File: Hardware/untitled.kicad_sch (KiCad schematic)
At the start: 11 parts, among them J7 Solar panel input, U1 MCP16311

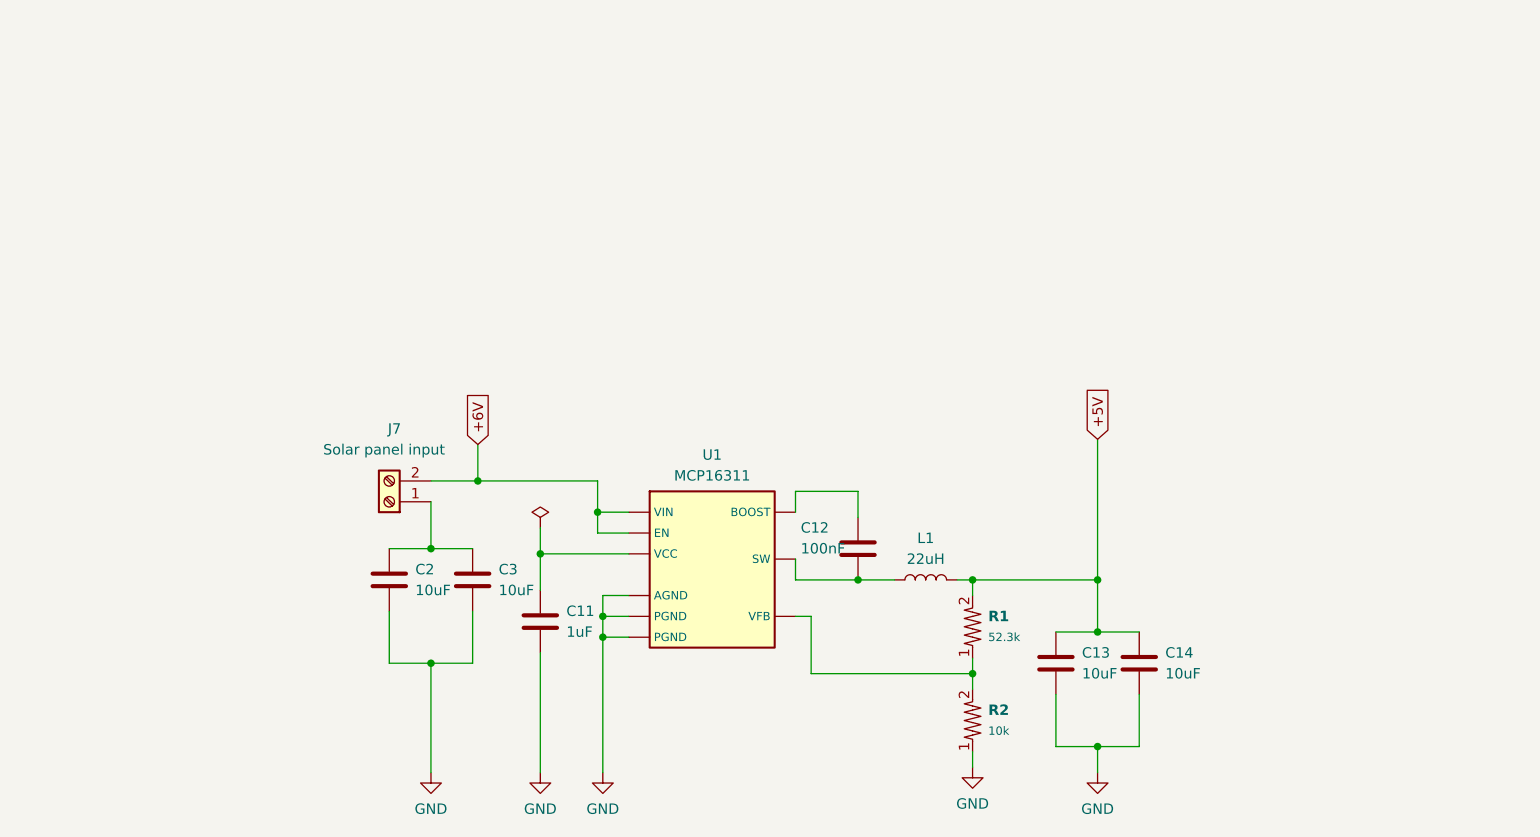
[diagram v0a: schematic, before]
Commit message: CHECK
CHECK1
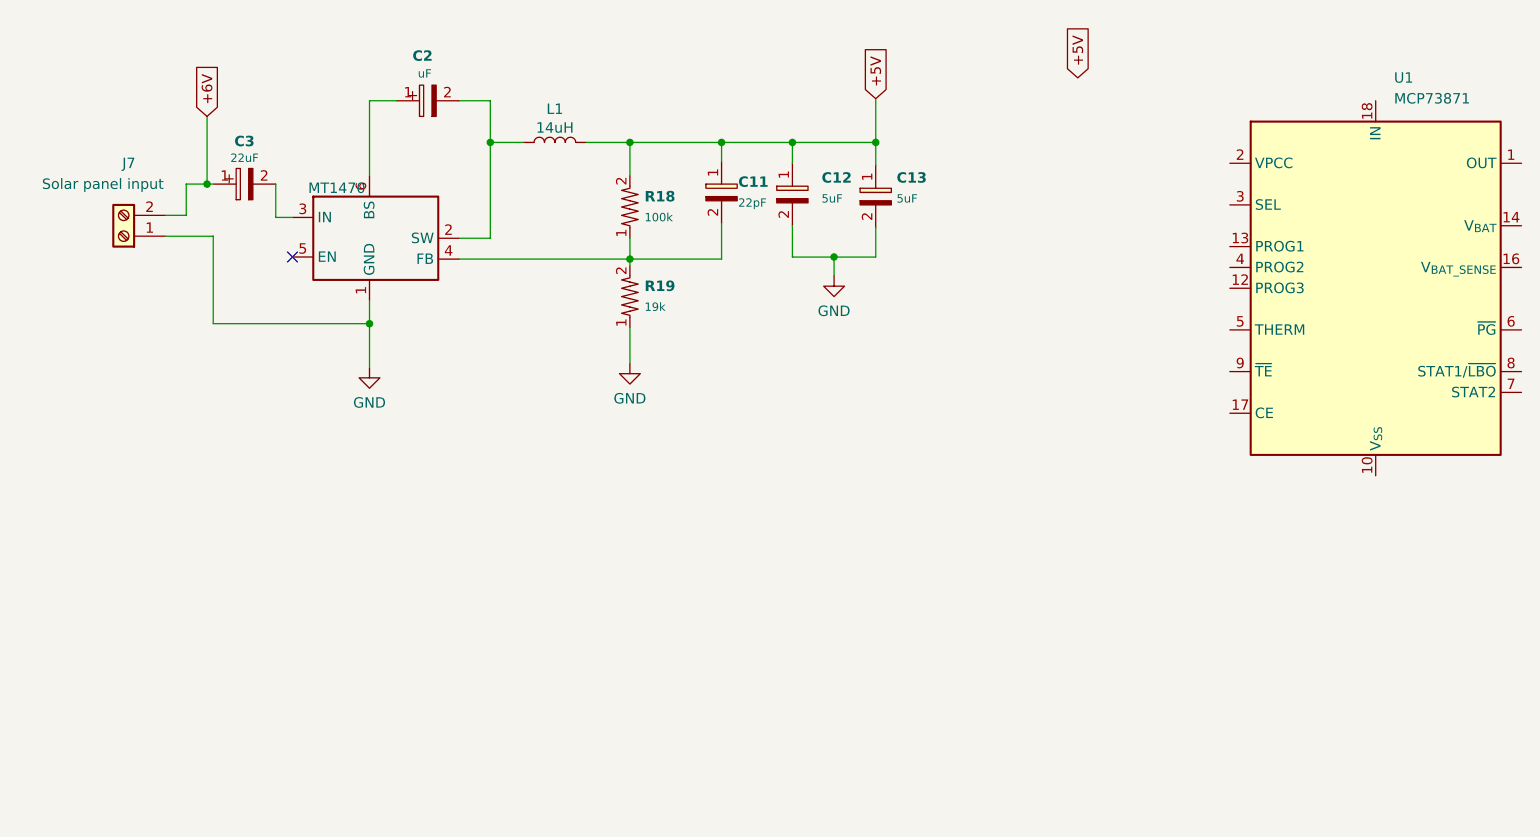
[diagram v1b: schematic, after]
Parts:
- removed C11: 1uF, symbol Device:C
- removed C12: 100nF, symbol Device:C
- removed C13, C14, C2, C3: 10uF, symbol Device:C
- removed R1: 52.3k, symbol Triet_KiCAD_Sym:Res
- removed R2: 10k, symbol Triet_KiCAD_Sym:Res
- removed U1: MCP16311, Triet_KiCAD_Fprint:MCP16311, symbol Triet_KiCAD_Sym:MCP16311
- added C11: 22pF, symbol Triet_KiCAD_Sym:CAP_CER
- added C12, C13: 5uF, symbol Triet_KiCAD_Sym:CAP_CER
- added C2: uF, symbol Triet_KiCAD_Sym:CAP_POL
- added C3: 22uF, symbol Triet_KiCAD_Sym:CAP_POL
- added MT1470: ~, symbol thinh:MT1470
- added R18: 100k, symbol Triet_KiCAD_Sym:Res
- added R19: 19k, symbol Triet_KiCAD_Sym:Res
- added U1: MCP73871, Package_DFN_QFN:QFN-20-1EP_4x4mm_P0.5mm_EP2.5x2.5mm, symbol Battery_Management:MCP73871
- L1: value 22uH -> 14uH
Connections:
- net +5V: now also C11.1, C12.1, C13.1, R18.2
- net +6V: now also C3.1
- net GND: now also J7.1 (Pin_1), C12.2, C13.2, MT1470.1 (GND), R19.1
- net at L1.1: now also C2.2, MT1470.2 (SW)
- new net: C3.2, MT1470.3 (IN)
- new net: C11.2, MT1470.4 (FB), R18.1, R19.2
- new net: C2.1, MT1470.6 (BS)
- new net: U1.1 (OUT), U1.20 (OUT)
- new net: U1.10 (V_{SS}), U1.11 (V_{SS}), U1.21 (V_{SS})
- new net: U1.14 (V_{BAT}), U1.15 (V_{BAT})
- new net: U1.18 (IN), U1.19 (IN)
- no-connect marks 0 -> 1
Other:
- moved on the sheet: J7

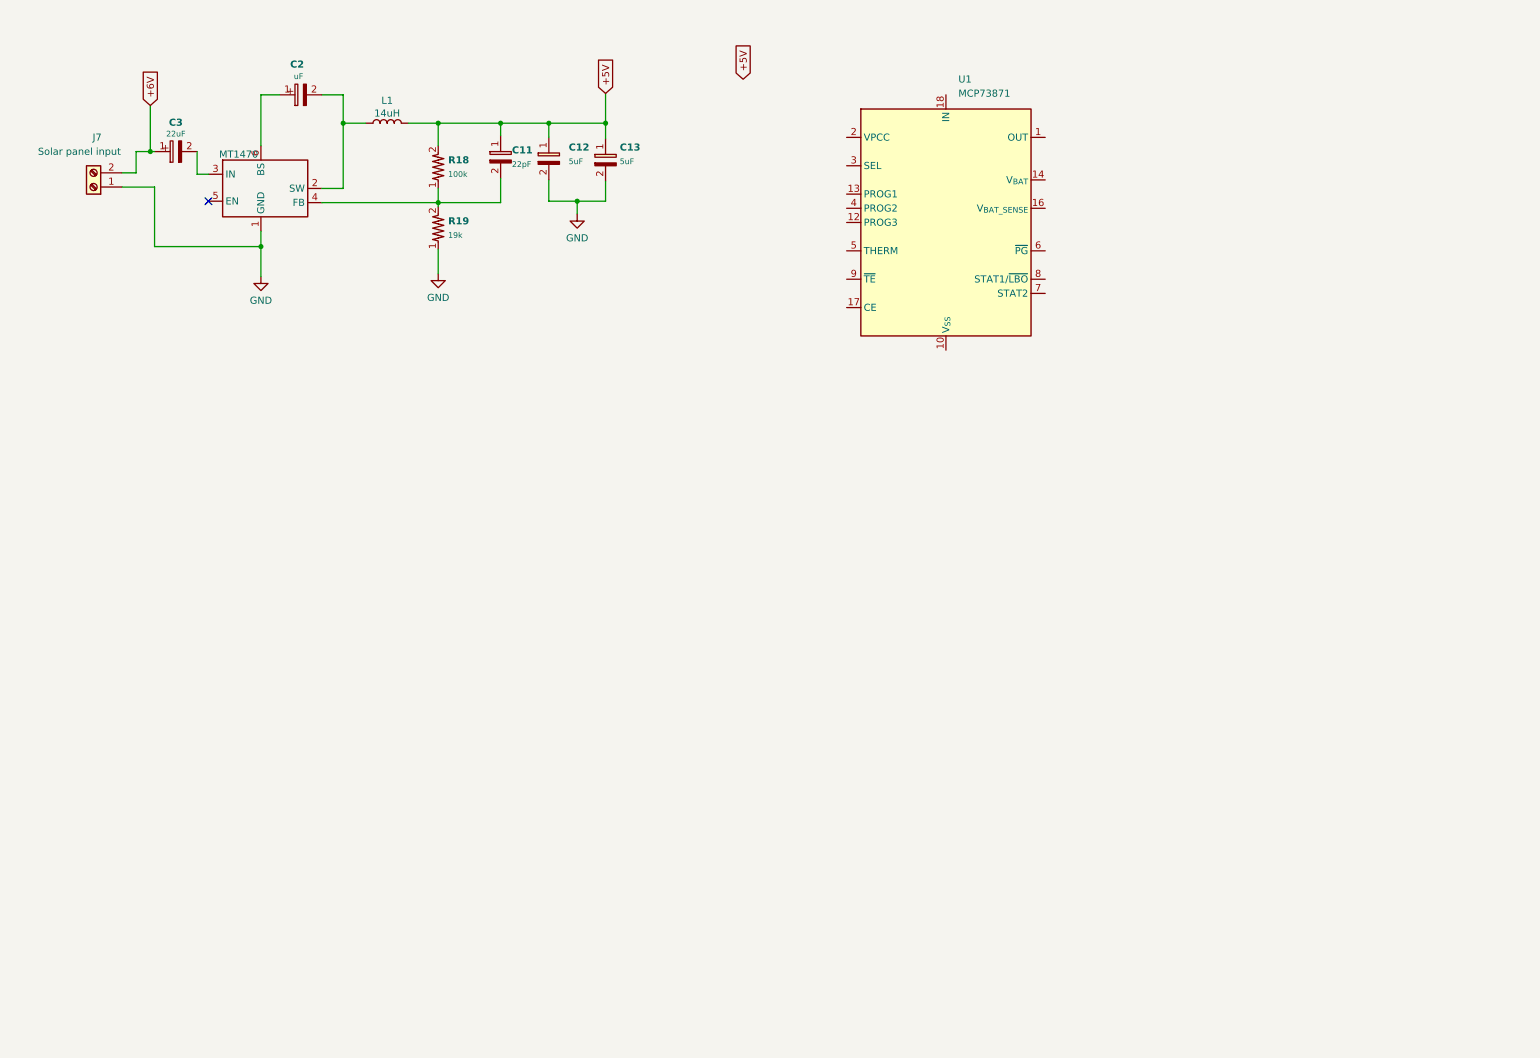
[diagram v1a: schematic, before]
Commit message: CHECK
CHECK
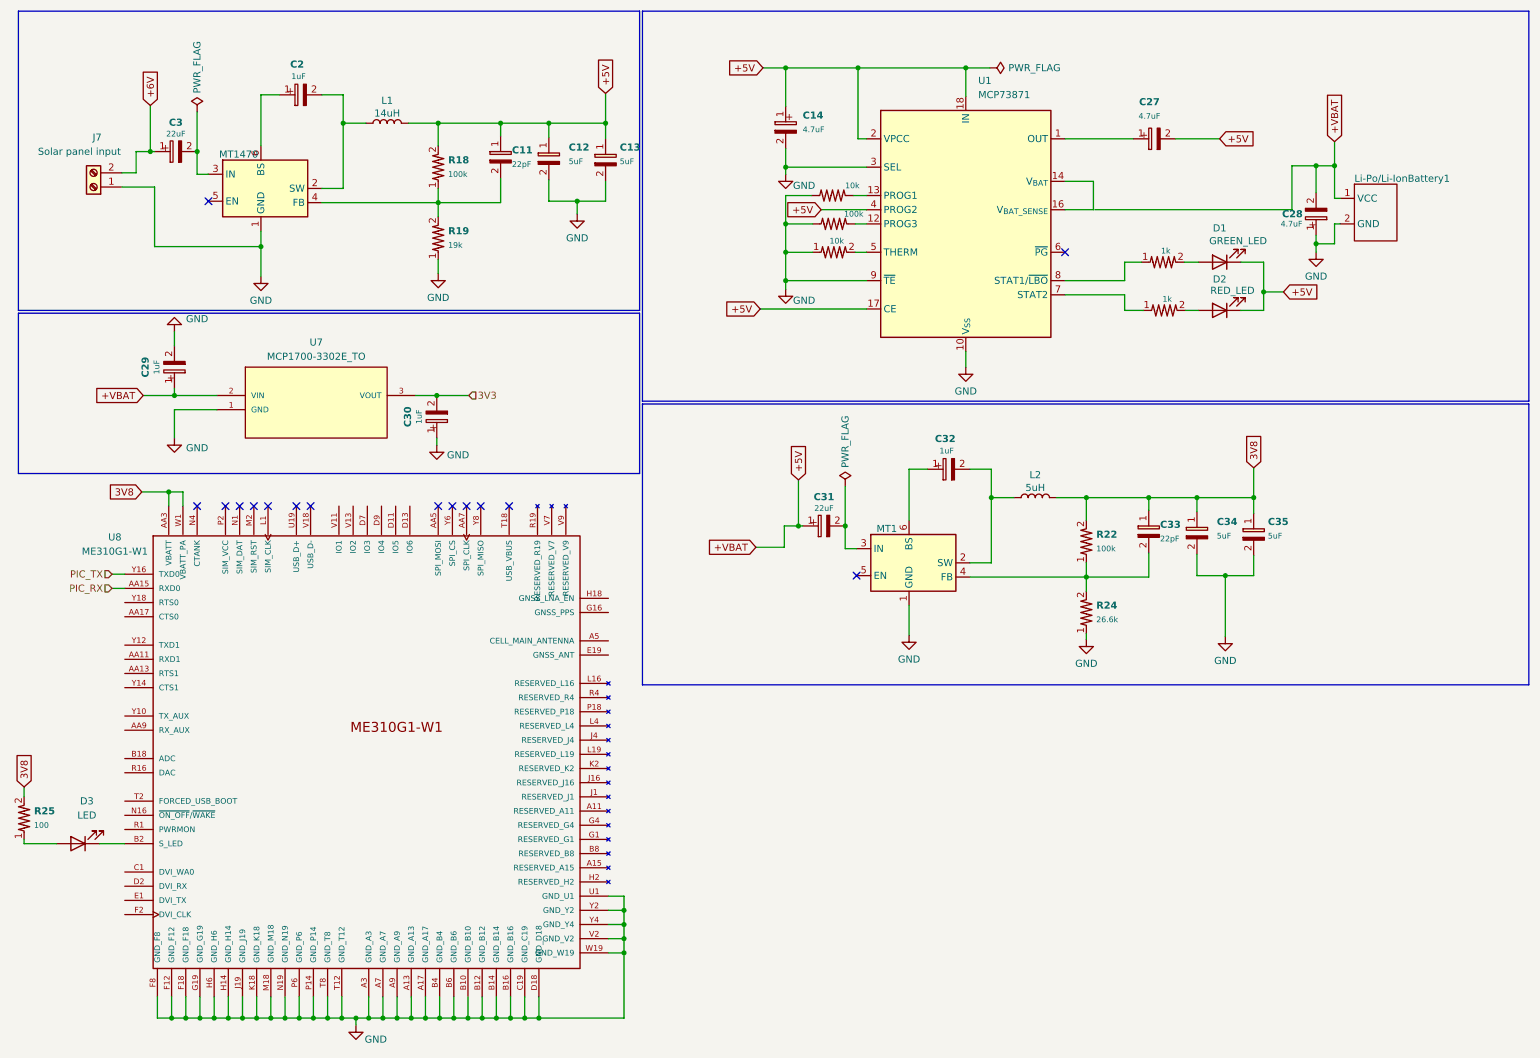
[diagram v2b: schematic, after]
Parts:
- added C14, C27, C28: 4.7uF, symbol Triet_KiCAD_Sym:CAP_POL
- added C29, C30, C32: 1uF, symbol Triet_KiCAD_Sym:CAP_POL
- added C31: 22uF, symbol Triet_KiCAD_Sym:CAP_POL
- added C33: 22pF, symbol Triet_KiCAD_Sym:CAP_CER
- added C34, C35: 5uF, symbol Triet_KiCAD_Sym:CAP_CER
- added D1: GREEN_LED, symbol Device:LED
- added D2: RED_LED, symbol Device:LED
- added D3: LED, symbol Device:LED
- added L2: 5uH, symbol Device:L
- added Li-Po/Li-IonBattery1: ~, symbol thinh:Li-Po/Li-Ion_Battery
- added MT1: ~, symbol thinh:MT1470
- added R17, R21: 1k, symbol Triet_KiCAD_Sym:Res
- added R2, R22: 100k, symbol Triet_KiCAD_Sym:Res
- added R20, R23: 10k, symbol Triet_KiCAD_Sym:Res
- added R24: 26.6k, symbol Triet_KiCAD_Sym:Res
- added R25: 100, symbol Triet_KiCAD_Sym:Res
- added U7: MCP1700-3302E_TO, symbol MCP1700:MCP1700-3302E_TO
- added U8: ME310G1-W1, symbol ME310G1-W1:ME310G1-W1
- C2: value uF -> 1uF
- U1: footprint Package_DFN_QFN:QFN-20-1EP_4x4mm_P0.5mm_EP2.5x2.5mm -> (none)
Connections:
- net +5V: now also U1.17 (CE), U1.18 (IN), U1.19 (IN), U1.2 (VPCC), U1.4 (PROG2), C14.1, C27.2, C28.2, C29.1, C31.1, D1.1 (K), D2.1 (K), Li-Po/Li-IonBattery1.1 (VCC), U7.2 (VIN)
- net GND: now also U1.10 (V_{SS}), U1.11 (V_{SS}), U1.21 (V_{SS}), U1.3 (SEL), U1.9 (~{TE}), C14.2, C28.1, C29.2, C30.1, C34.2, C35.2, Li-Po/Li-IonBattery1.2 (GND), MT1.1 (GND), R2.1, R20.1, R23.1, R24.1, U7.1 (GND), U8.A13 (GND_A13), U8.A17 (GND_A17), U8.A3 (GND_A3), U8.A7 (GND_A7), U8.A9 (GND_A9), U8.B10 (GND_B10), U8.B12 (GND_B12), U8.B14 (GND_B14), U8.B16 (GND_B16), U8.B4 (GND_B4), U8.B6 (GND_B6), U8.C19 (GND_C19), U8.D18 (GND_D18), U8.F12 (GND_F12), U8.F18 (GND_F18), U8.F8 (GND_F8), U8.G19 (GND_G19), U8.H14 (GND_H14), U8.H6 (GND_H6), U8.J19 (GND_J19), U8.K18 (GND_K18), U8.M18 (GND_M18), U8.N19 (GND_N19), U8.P14 (GND_P14), U8.P6 (GND_P6), U8.T12 (GND_T12), U8.T8 (GND_T8), U8.U1 (GND_U1), U8.V2 (GND_V2), U8.W19 (GND_W19), U8.Y2 (GND_Y2), U8.Y4 (GND_Y4)
- net at U1.1 (OUT): now also C27.1; no longer U1.20 (OUT)
- net at U1.12 (PROG3): now also R2.2
- net at U1.13 (PROG1): now also R23.2
- net at U1.14 (V_{BAT}), U1.15 (V_{BAT}): now also U1.16 (V_{BAT_SENSE})
- net at U1.5 (THERM): now also R20.2
- net at U1.7 (STAT2): now also R21.1
- net at U1.8 (STAT1/~{LBO}): now also R17.1
- new net: D3.1 (K), U8.B2 (S_LED)
- new net: C31.2, MT1.3 (IN)
- new net: C32.1, MT1.6 (BS)
- new net: C32.2, L2.1, MT1.2 (SW)
- new net: D1.2 (A), R17.2
- new net: C33.2, MT1.4 (FB), R22.1, R24.2
- new net: D2.2 (A), R21.2
- new net: D3.2 (A), R25.1
- new net 3V3: C30.2, U7.3 (VOUT)
- new net 3V8: C33.1, C34.1, C35.1, L2.2, R22.2, R25.2, U8.AA3 (VBATT), U8.W1 (VBATT_PA)
- new net PIC_RX: U8.AA15 (RXD0)
- new net PIC_TX: U8.Y16 (TXD0)
- no-connect marks 1 -> 15
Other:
- moved on the sheet: R19, U1
